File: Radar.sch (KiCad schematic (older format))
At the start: 13 parts, among them J1 Receive_Antenna, J2 VCO_Tune, J3 Transmit Antenna, J4 Output, U1 LNA_1, U2 SW1, U3 LNA_2, U4 VCO, U5 SW2, U6 PA, U7 mixer_diagram, U8 PGA, U9 lowpass_diagram

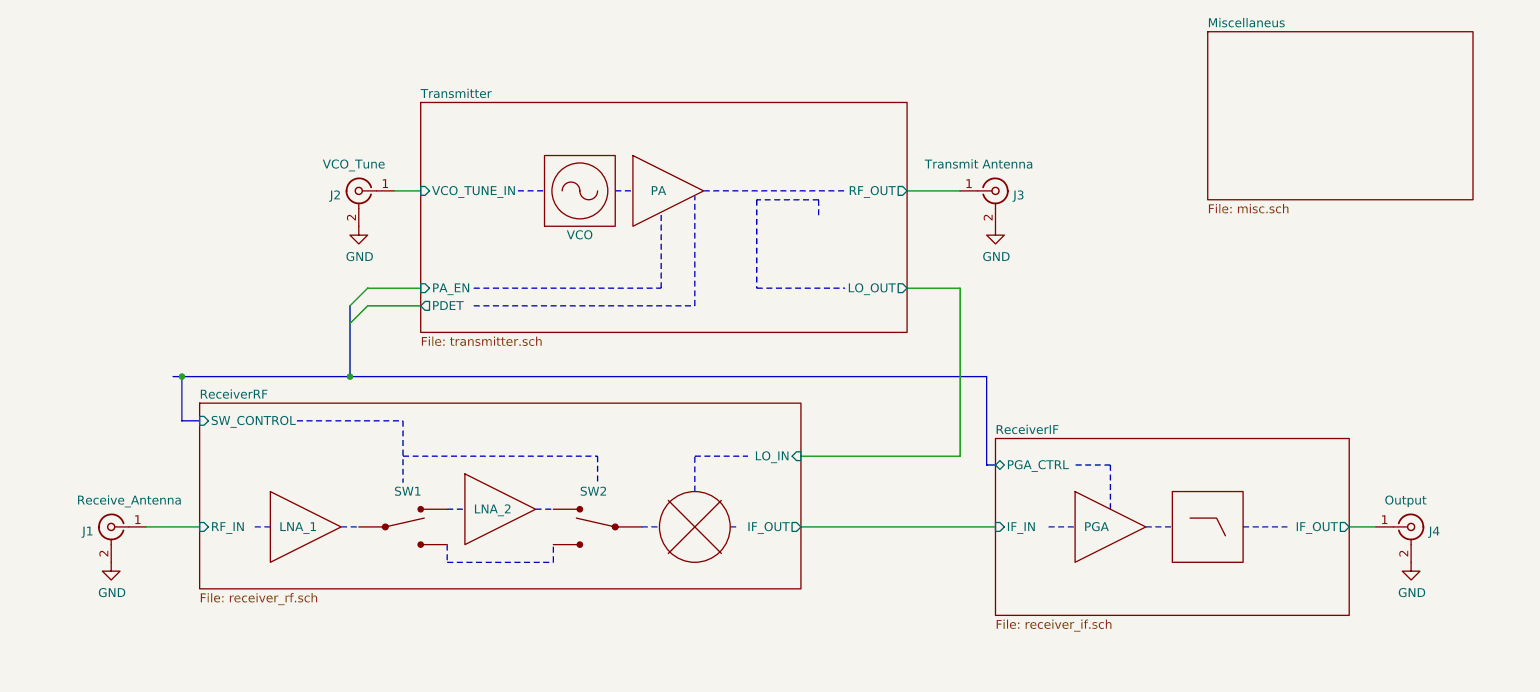
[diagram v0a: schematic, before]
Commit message: Schematic finishing touches
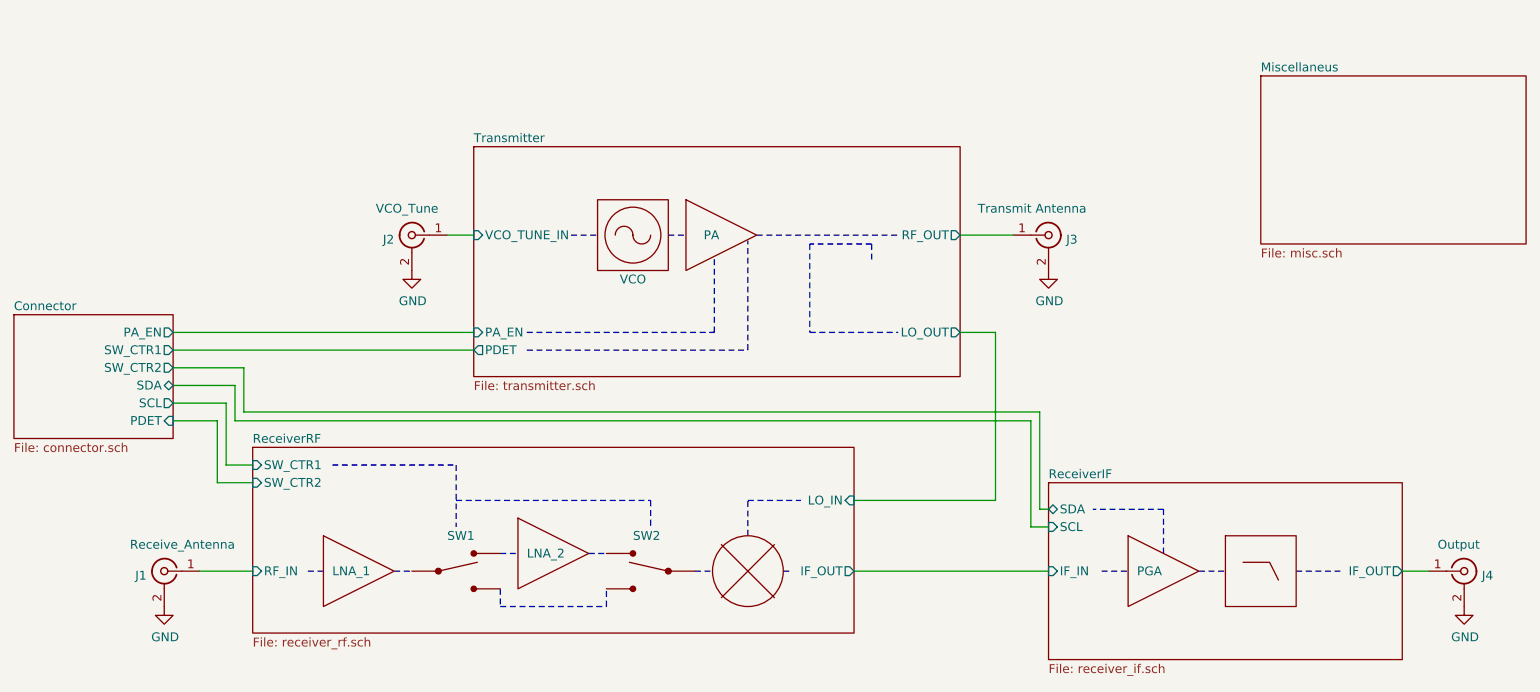
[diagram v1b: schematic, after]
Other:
- moved on the sheet: J1, J2, J3, J4
